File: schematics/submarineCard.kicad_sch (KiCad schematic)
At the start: 14 parts, among them U2 3MP SPI Camera, U4 MPU-6050

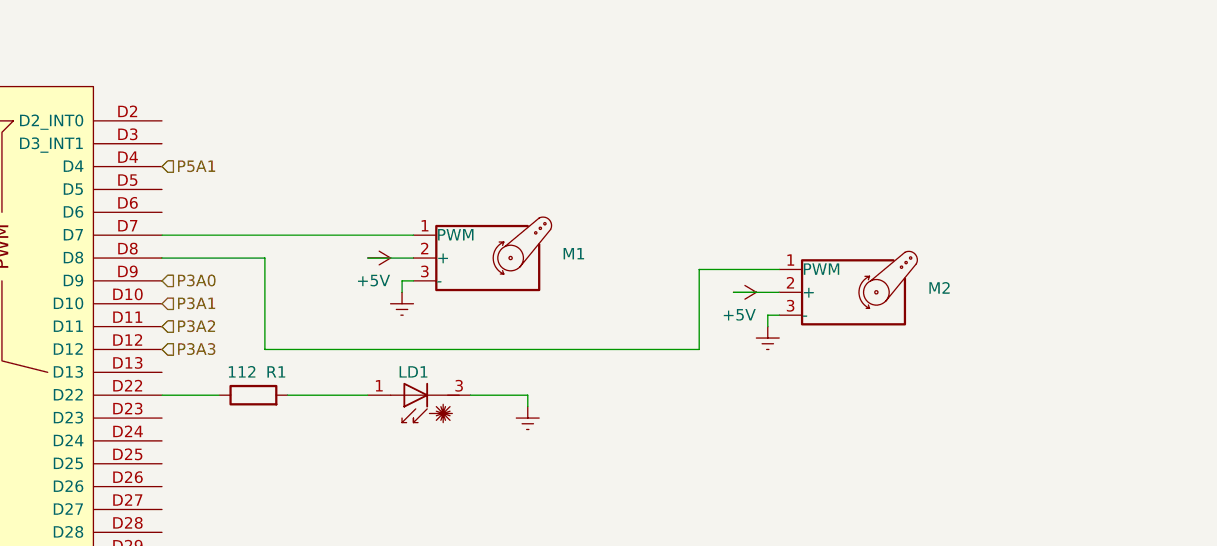
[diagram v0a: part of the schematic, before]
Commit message: new motor
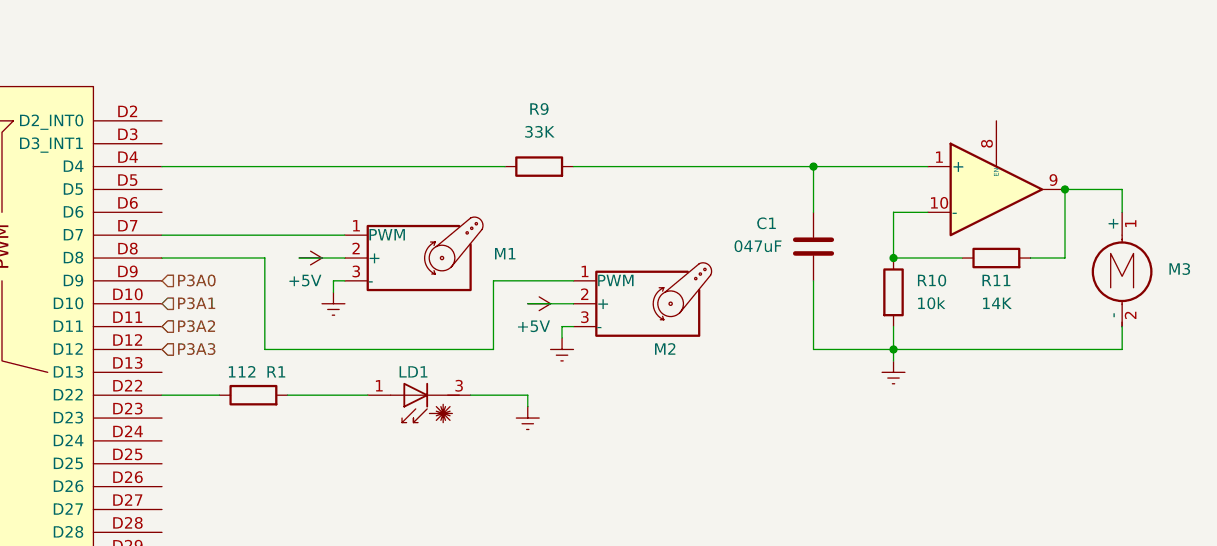
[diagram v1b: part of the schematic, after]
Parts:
- added C1: 047uF, symbol Device:C
- added M3: Motor_DC, symbol Motor:Motor_DC
- added R10: 10k, symbol Device:R
- added R11: 14K, symbol Device:R
- added R9: 33K, symbol Device:R
- added U1: OPA1622, Package_SON:Texas_S-PVSON-N10, symbol Amplifier_Audio:OPA1622
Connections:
- net Earth: now also C1.2, M3.2 (-), R10.2
- net P5A1: no longer names the net of A3.D4
- net P5A1: now also R9.1
- new net: R10.1, R11.1, U1.10 (-)
- new net: M3.1 (+), R11.2, U1.9
- new net: C1.1, R9.2, U1.1 (+)
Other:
- moved on the sheet: M1, M2
